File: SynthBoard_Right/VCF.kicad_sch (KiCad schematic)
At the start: 28 parts, among them U2 LM13700, U5 LM13700

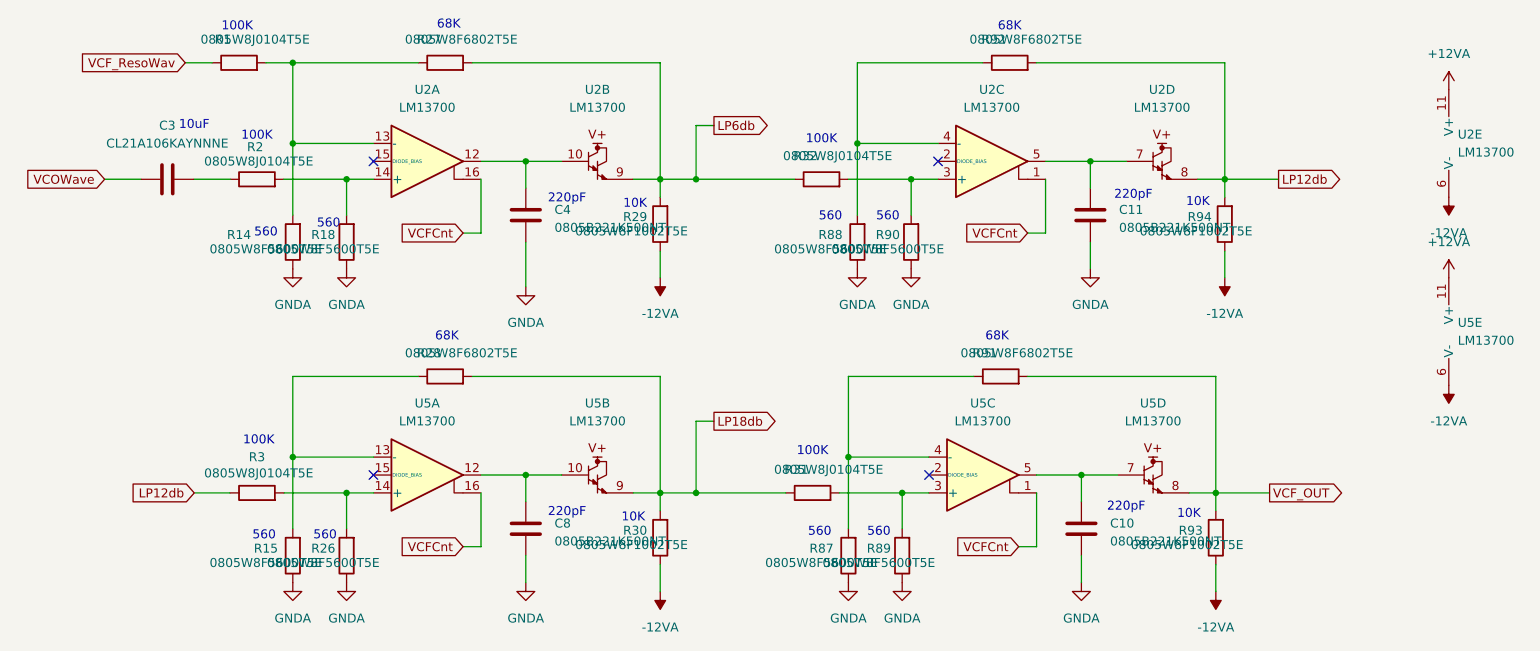
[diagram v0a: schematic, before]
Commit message: SynthBoard Right
Basic部品で更新まで
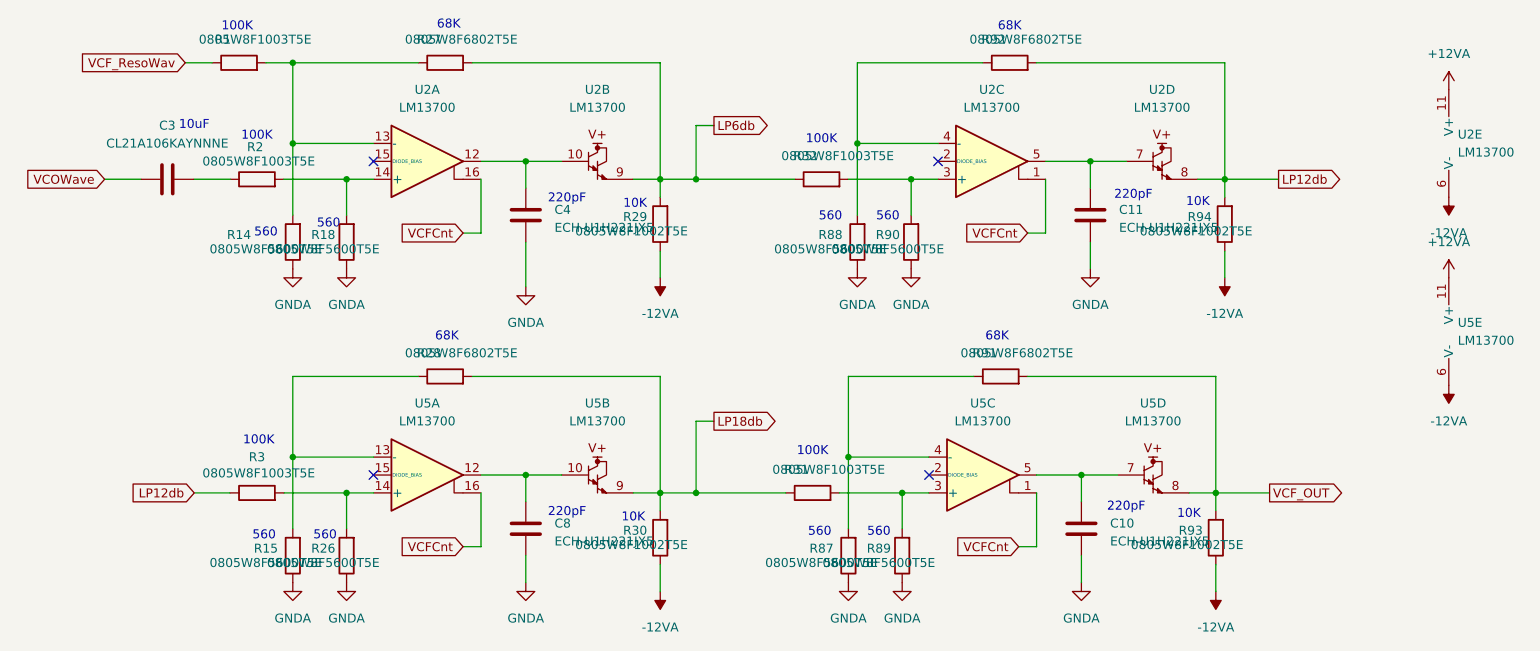
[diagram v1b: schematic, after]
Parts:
- C10, C11, C4, C8: value 0805B221K500NT -> ECH-U1H221JX5
- R1, R2, R3, R31, R32: value 0805W8J0104T5E -> 0805W8F1003T5E
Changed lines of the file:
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@@
 			)
 		)
-		(property "Value" "0805W8J0104T5E"
+		(property "Value" "0805W8F1003T5E"
 			(at 85.344 40.64 90)
 			(effects
@@
 			)
 		)
-		(property "Value" "0805B221K500NT"
+		(property "Value" "ECH-U1H221JX5"
 			(at 205.994 94.488 0)
 			(effects
@@
 			)
 		)
-		(property "Value" "0805W8J0104T5E"
+		(property "Value" "0805W8F1003T5E"
 			(at 84.836 23.368 90)
 			(effects
@@
 			)
 		)
-		(property "Value" "0805W8J0104T5E"
+		(property "Value" "0805W8F1003T5E"
 			(at 166.116 84.328 90)
 			(effects
@@
 			)
 		)
-		(property "Value" "0805B221K500NT"
+		(property "Value" "ECH-U1H221JX5"
 			(at 207.264 50.038 0)
 			(effects
@@
 			)
 		)
-		(property "Value" "0805B221K500NT"
+		(property "Value" "ECH-U1H221JX5"
 			(at 127.254 50.038 0)
 			(effects
@@
 			)
 		)
-		(property "Value" "0805W8J0104T5E"
+		(property "Value" "0805W8F1003T5E"
 			(at 167.386 39.878 90)
 			(effects
@@
 			)
 		)
-		(property "Value" "0805W8J0104T5E"
+		(property "Value" "0805W8F1003T5E"
 			(at 85.344 84.836 90)
 			(effects
@@
 			)
 		)
-		(property "Value" "0805B221K500NT"
+		(property "Value" "ECH-U1H221JX5"
 			(at 127.254 94.488 0)
 			(effects
